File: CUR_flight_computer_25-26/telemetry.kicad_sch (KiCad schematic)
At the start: 10 parts, among them U4 Ai-Thinker-Ra-01, U9 E22-400M30S

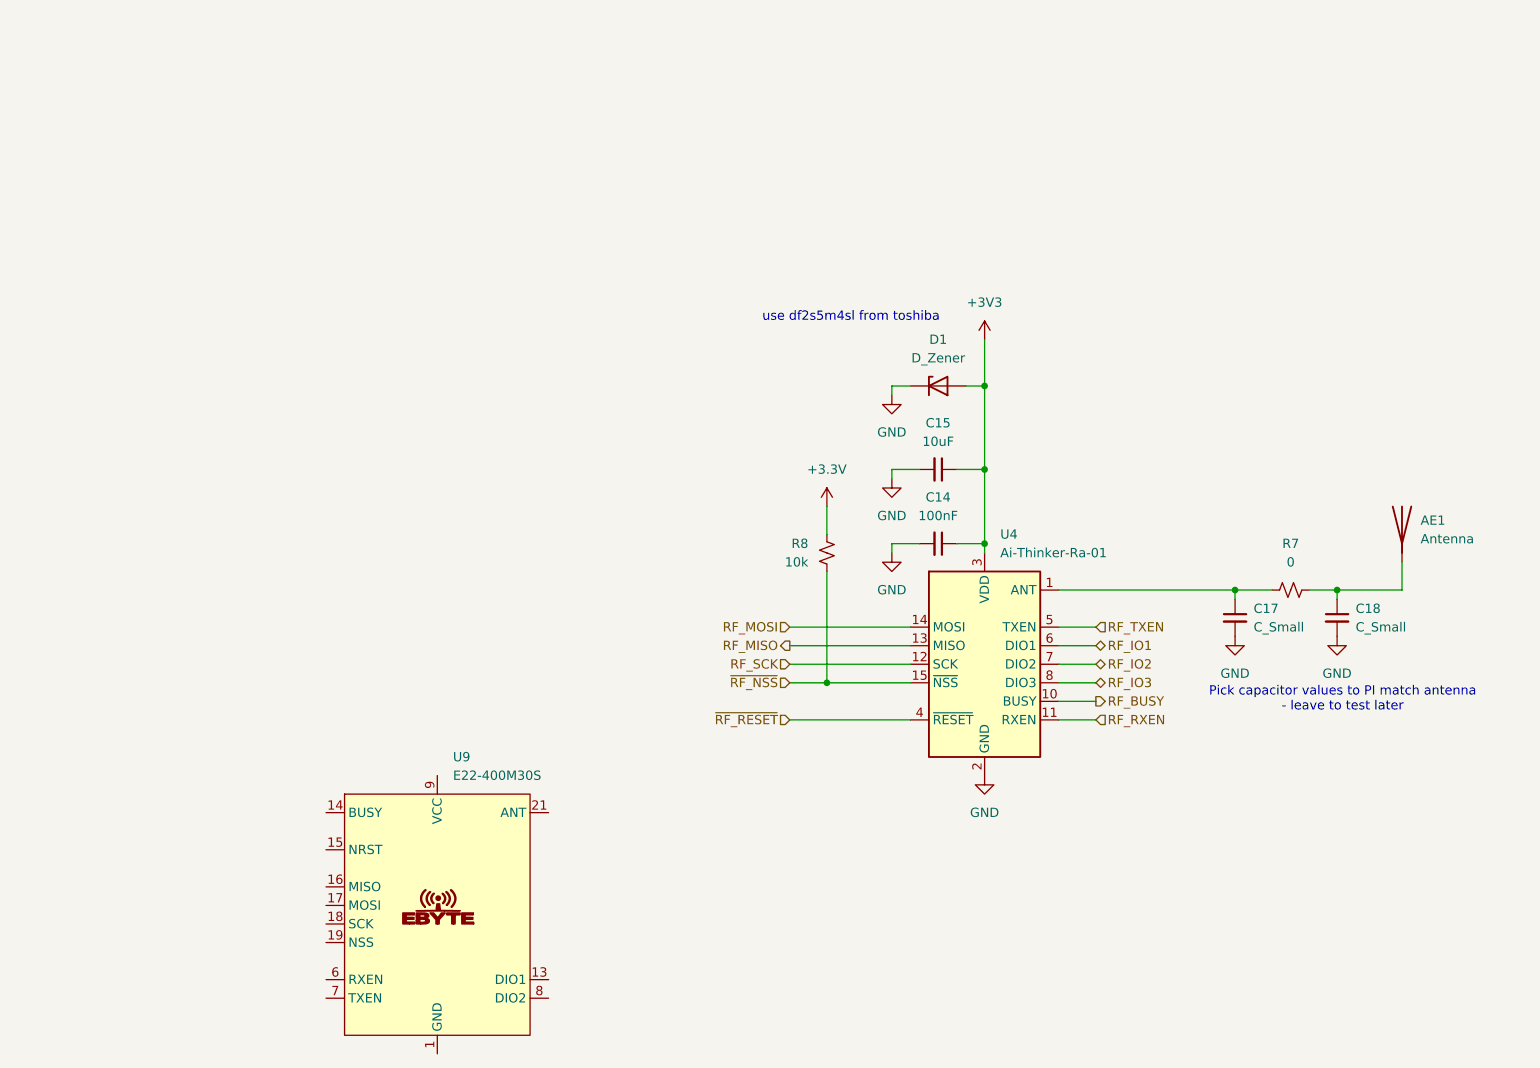
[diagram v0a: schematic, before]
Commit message: Update telemetry.kicad_sch
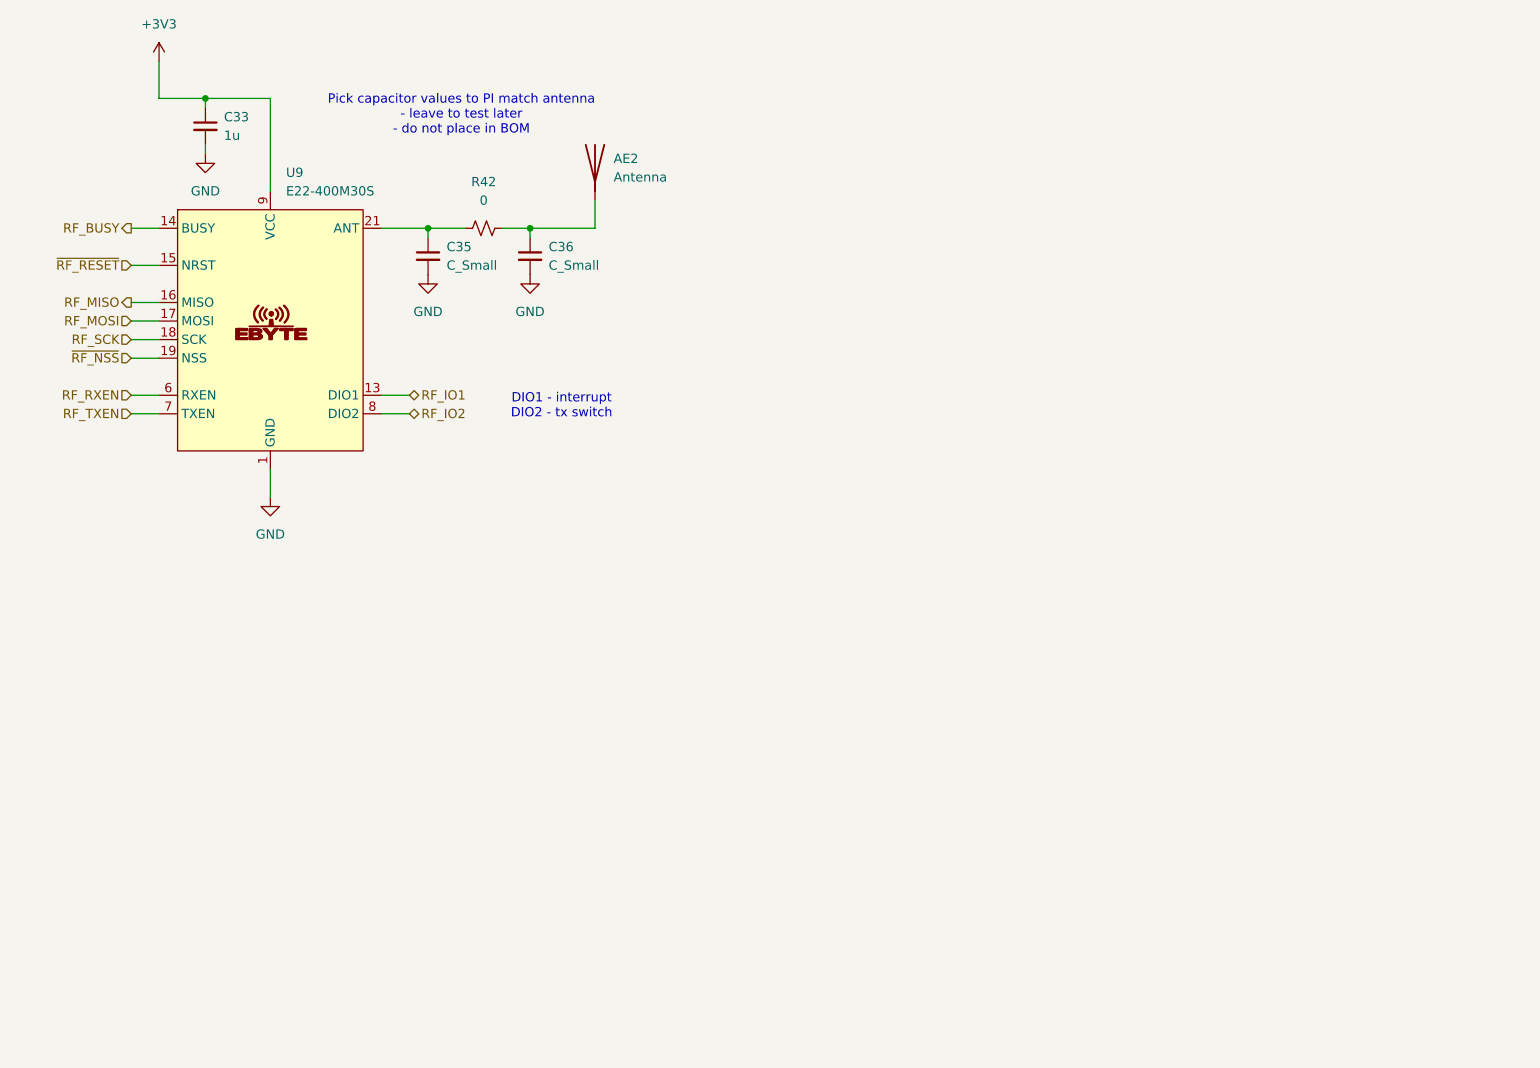
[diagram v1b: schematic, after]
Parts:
- removed AE1: Antenna, symbol Device:Antenna
- removed C14: 100nF, symbol Device:C_Small
- removed C15: 10uF, symbol Device:C_Small
- removed C17, C18: C_Small, symbol Device:C_Small
- removed D1: D_Zener, symbol Device:D_Zener
- removed R7: 0, symbol Device:R_Small_US
- removed R8: 10k, symbol Device:R_Small_US
- removed U4: Ai-Thinker-Ra-01, RF_Module:Ai-Thinker-Ra-01-LoRa, symbol RF_Module:Ai-Thinker-Ra-01
- added AE2: Antenna, symbol Device:Antenna
- added C33: 1u, symbol Device:C_Small
- added C35, C36: C_Small, symbol Device:C_Small
- added R42: 0, symbol Device:R_Small_US
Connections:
- net VCC is gone; now on net +3V3: U9.10 (VCC), U9.9 (VCC)
- net +3V3: now also C33.1
- net GND: now also C33.2, C35.2, C36.2
- net RF_BUSY: now also U9.14 (BUSY)
- net RF_IO1: now also U9.13 (DIO1)
- net RF_IO2: now also U9.8 (DIO2)
- net RF_MISO: now also U9.16 (MISO)
- net RF_MOSI: now also U9.17 (MOSI)
- net RF_RXEN: now also U9.6 (RXEN)
- net RF_SCK: now also U9.18 (SCK)
- net RF_TXEN: now also U9.7 (TXEN)
- net ~{RF_NSS}: now also U9.19 (NSS)
- net ~{RF_RESET}: now also U9.15 (NRST)
- net at U9.21 (ANT): now also C35.1, R42.2
- new net: AE2.1 (A), C36.1, R42.1
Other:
- note added: "DIO1 - interrupt DIO2 - tx switch"
- note added: "Pick capacitor values to PI match antenna - leave to test later - do not place in BOM"
- note removed: "Pick capacitor values to PI match antenna - leave to test later"
- note removed: "use df2s5m4sl from toshiba"
- moved on the sheet: U9
